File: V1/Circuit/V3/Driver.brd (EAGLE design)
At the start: 61 x 56 mm, 37 parts, among them IC1 DRV8303DCA

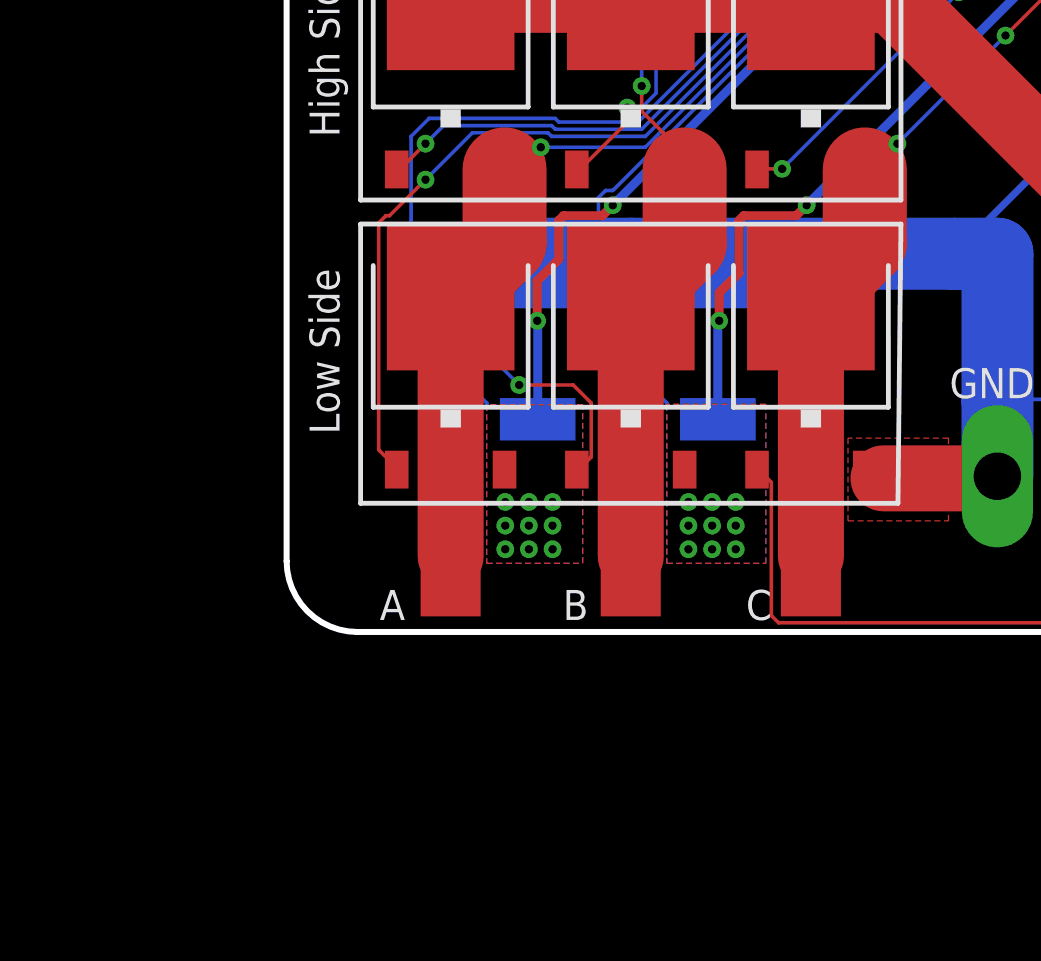
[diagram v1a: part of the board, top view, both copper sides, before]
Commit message: Circuit: Added DRV8300, and the Gate Circuit. Haven't added the Not gate
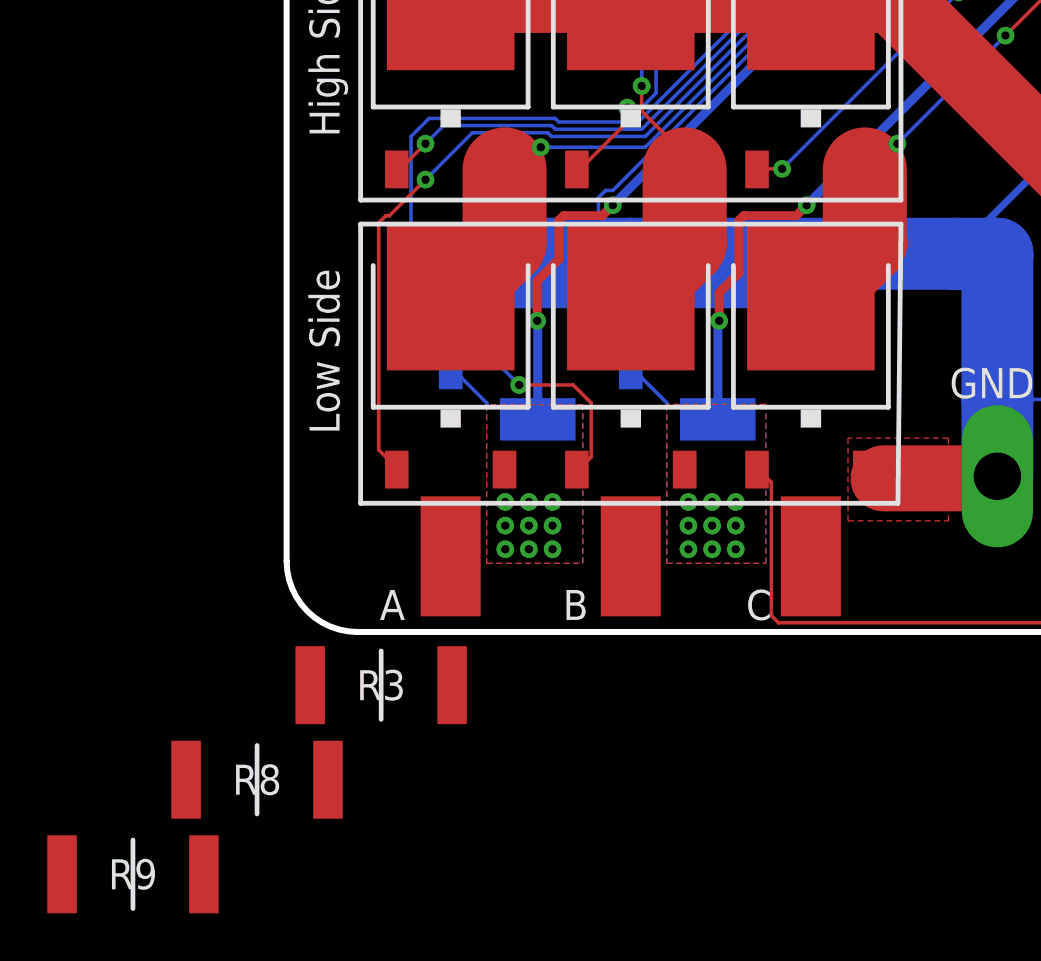
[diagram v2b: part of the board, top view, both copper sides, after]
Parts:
- added R3, R8, R9: CR2512-FX-51R1ELF, CR2512-FX-51R1ELF:RESC6331X75N
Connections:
- new net N$5: HA.2, LA.3, R3.2
- new net N$6: B.1, R8.1
- new net N$7: HC.2, LC.3, R9.2
- net SH_A: now also R3.1; no longer HA.2, LA.3
- net SH_B: now also R8.2; no longer B.1
- net SH_C: now also R9.1; no longer HC.2, LC.3
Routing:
- net SH_A: track 45.4 -> 25.1 mm
- net SH_C: track 38.6 -> 19.5 mm
- net SH_B: track 47.9 -> 37.0 mm
- net N$5: track 0.00 -> 7.56 mm
- net N$7: track 0.00 -> 6.34 mm
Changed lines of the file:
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@@
 <attribute name="VALUE" x="34.238" y="23.127" size="0.6096" layer="28" font="vector" ratio="20" rot="MR90" align="top-center"/>
+</element>
+<element name="R3" library="CR2512-FX-51R1ELF" package="RESC6331X75N" value="CR2512-FX-51R1ELF" x="3" y="-3.25" smashed="yes">
+<attribute name="ARROW_PART_NUMBER" value="CR2512-FX-51R1ELF" x="3" y="-3.25" size="1.778" layer="27" display="off"/>
+<attribute name="ARROW_PRICE-STOCK" value="https://www.arrow.com/en/products/cr2512-fx-51r1elf/bourns" x="3" y="-3.25" size="1.778" layer="27" display="off"/>
+<attribute name="DESCRIPTION" value="BOURNS - CR2512-FX-51R1ELF - RES 2512 51R1 1% 1W TC100 28X7511" x="3" y="-3.25" size="1.778" layer="27" display="off"/>
+<attribute name="HEIGHT" value="0.75mm" x="3" y="-3.25" size="1.778" layer="27" display="off"/>
+<attribute name="MANUFACTURER_NAME" value="Bourns" x="3" y="-3.25" size="1.778" layer="27" display="off"/>
+<attribute name="MANUFACTURER_PART_NUMBER" value="CR2512-FX-51R1ELF" x="3" y="-3.25" size="1.778" layer="27" display="off"/>
+<attribute name="MOUSER_PART_NUMBER" value="652-CR2512FX51R1ELF" x="3" y="-3.25" size="1.778" layer="27" display="off"/>
+<attribute name="MOUSER_PRICE-STOCK" value="https://www.mouser.com/Search/Refine.aspx?Keyword=652-CR2512FX51R1ELF" x="3" y="-3.25" size="1.778" layer="27" display="off"/>
+<attribute name="NAME" x="3" y="-3.25" size="1.27" layer="25" align="center"/>
+<attribute name="VALUE" x="3" y="-3.25" size="1.27" layer="27" align="center"/>
+</element>
+<element name="R8" library="CR2512-FX-51R1ELF" package="RESC6331X75N" value="CR2512-FX-51R1ELF" x="-2.25" y="-7.25" smashed="yes">
+<attribute name="ARROW_PART_NUMBER" value="CR2512-FX-51R1ELF" x="-2.25" y="-7.25" size="1.778" layer="27" display="off"/>
+<attribute name="ARROW_PRICE-STOCK" value="https://www.arrow.com/en/products/cr2512-fx-51r1elf/bourns" x="-2.25" y="-7.25" size="1.778" layer="27" display="off"/>
+<attribute name="DESCRIPTION" value="BOURNS - CR2512-FX-51R1ELF - RES 2512 51R1 1% 1W TC100 28X7511" x="-2.25" y="-7.25" size="1.778" layer="27" display="off"/>
+<attribute name="HEIGHT" value="0.75mm" x="-2.25" y="-7.25" size="1.778" layer="27" display="off"/>
+<attribute name="MANUFACTURER_NAME" value="Bourns" x="-2.25" y="-7.25" size="1.778" layer="27" display="off"/>
+<attribute name="MANUFACTURER_PART_NUMBER" value="CR2512-FX-51R1ELF" x="-2.25" y="-7.25" size="1.778" layer="27" display="off"/>
+<attribute name="MOUSER_PART_NUMBER" value="652-CR2512FX51R1ELF" x="-2.25" y="-7.25" size="1.778" layer="27" display="off"/>
+<attribute name="MOUSER_PRICE-STOCK" value="https://www.mouser.com/Search/Refine.aspx?Keyword=652-CR2512FX51R1ELF" x="-2.25" y="-7.25" size="1.778" layer="27" display="off"/>
+<attribute name="NAME" x="-2.25" y="-7.25" size="1.27" layer="25" align="center"/>
+<attribute name="VALUE" x="-2.25" y="-7.25" size="1.27" layer="27" align="center"/>
+</element>
+<element name="R9" library="CR2512-FX-51R1ELF" package="RESC6331X75N" value="CR2512-FX-51R1ELF" x="-7.5" y="-11.25" smashed="yes">
+<attribute name="ARROW_PART_NUMBER" value="CR2512-FX-51R1ELF" x="-7.5" y="-11.25" size="1.778" layer="27" display="off"/>
+<attribute name="ARROW_PRICE-STOCK" value="https://www.arrow.com/en/products/cr2512-fx-51r1elf/bourns" x="-7.5" y="-11.25" size="1.778" layer="27" display="off"/>
+<attribute name="DESCRIPTION" value="BOURNS - CR2512-FX-51R1ELF - RES 2512 51R1 1% 1W TC100 28X7511" x="-7.5" y="-11.25" size="1.778" layer="27" display="off"/>
+<attribute name="HEIGHT" value="0.75mm" x="-7.5" y="-11.25" size="1.778" layer="27" display="off"/>
+<attribute name="MANUFACTURER_NAME" value="Bourns" x="-7.5" y="-11.25" size="1.778" layer="27" display="off"/>
+<attribute name="MANUFACTURER_PART_NUMBER" value="CR2512-FX-51R1ELF" x="-7.5" y="-11.25" size="1.778" layer="27" display="off"/>
+<attribute name="MOUSER_PART_NUMBER" value="652-CR2512FX51R1ELF" x="-7.5" y="-11.25" size="1.778" layer="27" display="off"/>
+<attribute name="MOUSER_PRICE-STOCK" value="https://www.mouser.com/Search/Refine.aspx?Keyword=652-CR2512FX51R1ELF" x="-7.5" y="-11.25" size="1.778" layer="27" display="off"/>
+<attribute name="NAME" x="-7.5" y="-11.25" size="1.27" layer="25" align="center"/>
+<attribute name="VALUE" x="-7.5" y="-11.25" size="1.27" layer="27" align="center"/>
 </element>
 </elements>
@@
 </signal>
 <signal name="SH_C">
-<contactref element="HC" pad="2"/>
-<contactref element="LC" pad="3"/>
 <contactref element="C" pad="1"/>
 <contactref element="IC1" pad="32"/>
 <contactref element="C13" pad="2"/>
-<wire x1="21.18" y1="13.168" x2="21.18" y2="2.199" width="2.794" layer="1"/>
-<wire x1="23.46" y1="18.568" x2="23.46" y2="15.448" width="3.556" layer="1"/>
-<wire x1="23.46" y1="15.448" x2="21.18" y2="13.168" width="3.556" layer="1"/>
 <wire x1="33.8328" y1="28.956" x2="33.8328" y2="28.0416" width="0.1524" layer="16"/>
 <wire x1="33.6804" y1="29.1084" x2="33.8328" y2="28.956" width="0.1524" layer="16"/>
@@
 <wire x1="29.4132" y1="24.2316" x2="33.6804" y2="28.4988" width="0.1524" layer="1"/>
 <wire x1="24.8412" y1="19.6596" x2="29.4132" y2="24.2316" width="0.1524" layer="16"/>
-<wire x1="24.8412" y1="19.6596" x2="23.46" y2="18.568" width="0.1524" layer="1"/>
 <via x="33.6804" y="29.1084" extent="1-16" drill="0.35"/>
 <via x="32.004" y="32.3088" extent="1-16" drill="0.35"/>
 <via x="29.4132" y="24.2316" extent="1-16" drill="0.35"/>
 <via x="24.8412" y="19.6596" extent="1-16" drill="0.35"/>
+<contactref element="R9" pad="1"/>
+<wire x1="21.18" y1="2.199" x2="24.8412" y2="19.6596" width="0" layer="19" extent="1-1"/>
+<wire x1="-10.5" y1="-11.25" x2="21.18" y2="2.199" width="0" layer="19" extent="1-1"/>
 </signal>
 <signal name="GH_C">
@@
 <contactref element="HB" pad="2"/>
 <contactref element="LB" pad="3"/>
-<contactref element="B" pad="1"/>
 <contactref element="IC1" pad="37"/>
 <contactref element="C12" pad="2"/>
-<wire x1="13.56" y1="13.168" x2="13.56" y2="2.199" width="2.794" layer="1"/>
 <wire x1="15.84" y1="18.568" x2="15.84" y2="15.448" width="3.556" layer="1"/>
 <wire x1="15.84" y1="15.448" x2="13.56" y2="13.168" width="3.556" layer="1"/>
@@
 <wire x1="14.9352" y1="20.1168" x2="15.84" y2="18.568" width="0.1524" layer="1"/>
 <via x="14.0208" y="22.098" extent="1-16" drill="0.35"/>
+<contactref element="R8" pad="2"/>
+<wire x1="0.75" y1="-7.25" x2="13.56" y2="13.168" width="0" layer="19" extent="1-1"/>
 </signal>
 <signal name="SN2">
@@
 </signal>
 <signal name="SH_A">
-<contactref element="HA" pad="2"/>
-<contactref element="LA" pad="3"/>
 <contactref element="A" pad="1"/>
 <contactref element="IC1" pad="42"/>
 <contactref element="C1" pad="2"/>
-<wire x1="8.22" y1="18.568" x2="8.22" y2="15.47" width="3.556" layer="1"/>
-<wire x1="8.22" y1="15.47" x2="5.5" y2="12.75" width="3.556" layer="1"/>
-<wire x1="5.5" y1="12.75" x2="5.522" y2="12.75" width="3.556" layer="1"/>
-<wire x1="5.522" y1="12.75" x2="5.94" y2="13.168" width="3.556" layer="1"/>
-<wire x1="5.94" y1="13.168" x2="5.94" y2="2.199" width="2.794" layer="1"/>
 <wire x1="25.6032" y1="28.956" x2="25.6032" y2="28.0416" width="0.1524" layer="16"/>
 <wire x1="26.67" y1="30.0228" x2="25.908" y2="29.2608" width="0.1524" layer="16"/>
@@
 <wire x1="14.1732" y1="19.5072" x2="22.4028" y2="27.7368" width="0.1524" layer="16"/>
 <wire x1="9.7536" y1="19.5072" x2="14.1732" y2="19.5072" width="0.1524" layer="16"/>
-<wire x1="9.7536" y1="19.5072" x2="8.22" y2="18.568" width="0.1524" layer="1"/>
 <via x="25.908" y="29.1084" extent="1-16" drill="0.35"/>
 <via x="23.0124" y="29.5656" extent="1-16" drill="0.35"/>
 <via x="9.7536" y="19.5072" extent="1-16" drill="0.35"/>
+<contactref element="R3" pad="1"/>
+<wire x1="5.94" y1="2.199" x2="9.7536" y2="19.5072" width="0" layer="19" extent="1-1"/>
+<wire x1="0" y1="-3.25" x2="5.94" y2="2.199" width="0" layer="19" extent="1-1"/>
 </signal>
 <signal name="GH_A">
@@
 <via x="36.4236" y="36.1188" extent="1-16" drill="0.35"/>
 </signal>
+<signal name="N$5">
+<contactref element="HA" pad="2"/>
+<contactref element="LA" pad="3"/>
+<wire x1="8.22" y1="18.568" x2="8.22" y2="15.47" width="3.556" layer="1"/>
+<wire x1="8.22" y1="15.47" x2="5.5" y2="12.75" width="3.556" layer="1"/>
+<wire x1="5.5" y1="12.75" x2="5.522" y2="12.75" width="3.556" layer="1"/>
+<wire x1="5.522" y1="12.75" x2="5.94" y2="13.168" width="3.556" layer="1"/>
+<contactref element="R3" pad="2"/>
+<wire x1="6" y1="-3.25" x2="5.94" y2="13.168" width="0" layer="19" extent="1-1"/>
+</signal>
+<signal name="N$6">
+<contactref element="B" pad="1"/>
+<contactref element="R8" pad="1"/>
+<wire x1="-5.25" y1="-7.25" x2="13.56" y2="2.199" width="0" layer="19" extent="1-1"/>
+</signal>
+<signal name="N$7">
+<contactref element="HC" pad="2"/>
+<contactref element="LC" pad="3"/>
+<wire x1="23.46" y1="18.568" x2="23.46" y2="15.448" width="3.556" layer="1"/>
+<wire x1="23.46" y1="15.448" x2="21.18" y2="13.168" width="3.556" layer="1"/>
+<contactref element="R9" pad="2"/>
+<wire x1="-4.5" y1="-11.25" x2="21.18" y2="13.168" width="0" layer="19" extent="1-1"/>
+</signal>
 </signals>
